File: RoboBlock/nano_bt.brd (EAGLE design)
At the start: 100 x 80 mm, 17 parts, among them IC1 L293D, M1 ARDUINO-NANO-3.0

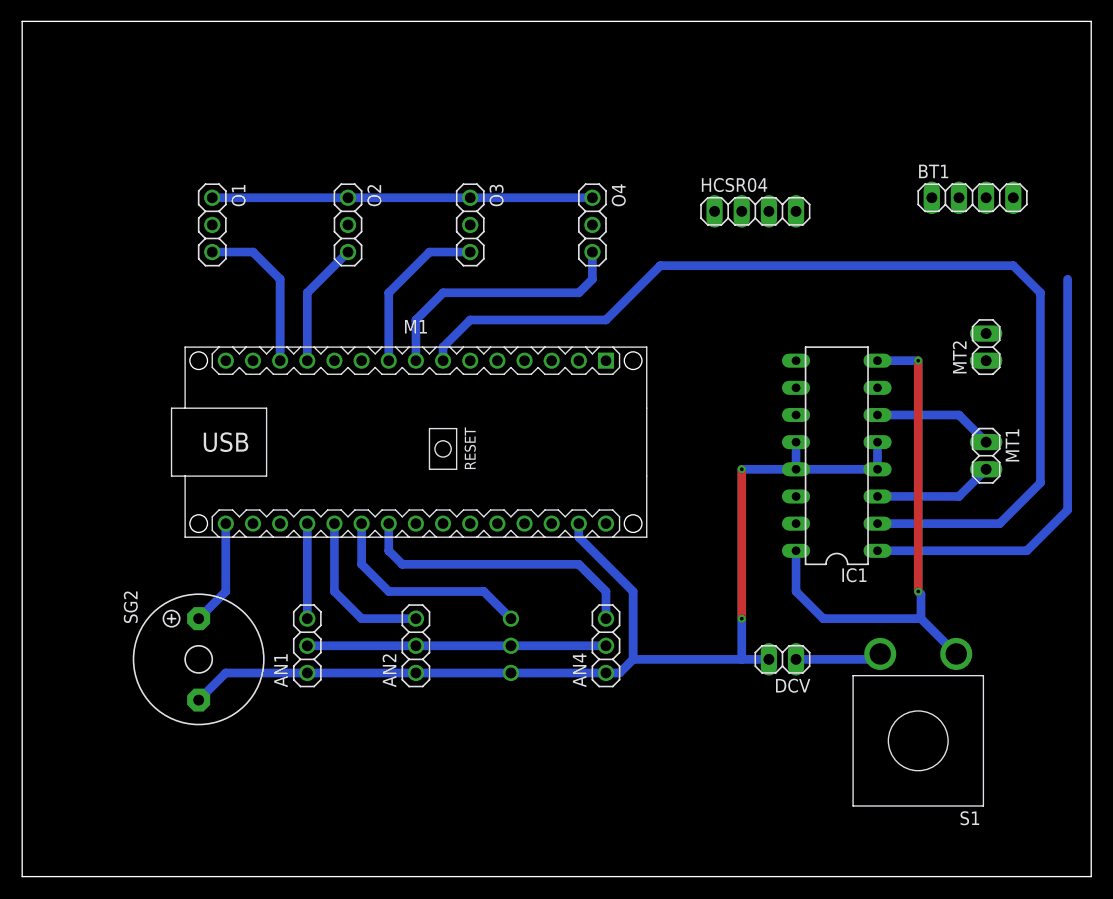
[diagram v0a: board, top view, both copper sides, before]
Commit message: printout pcb
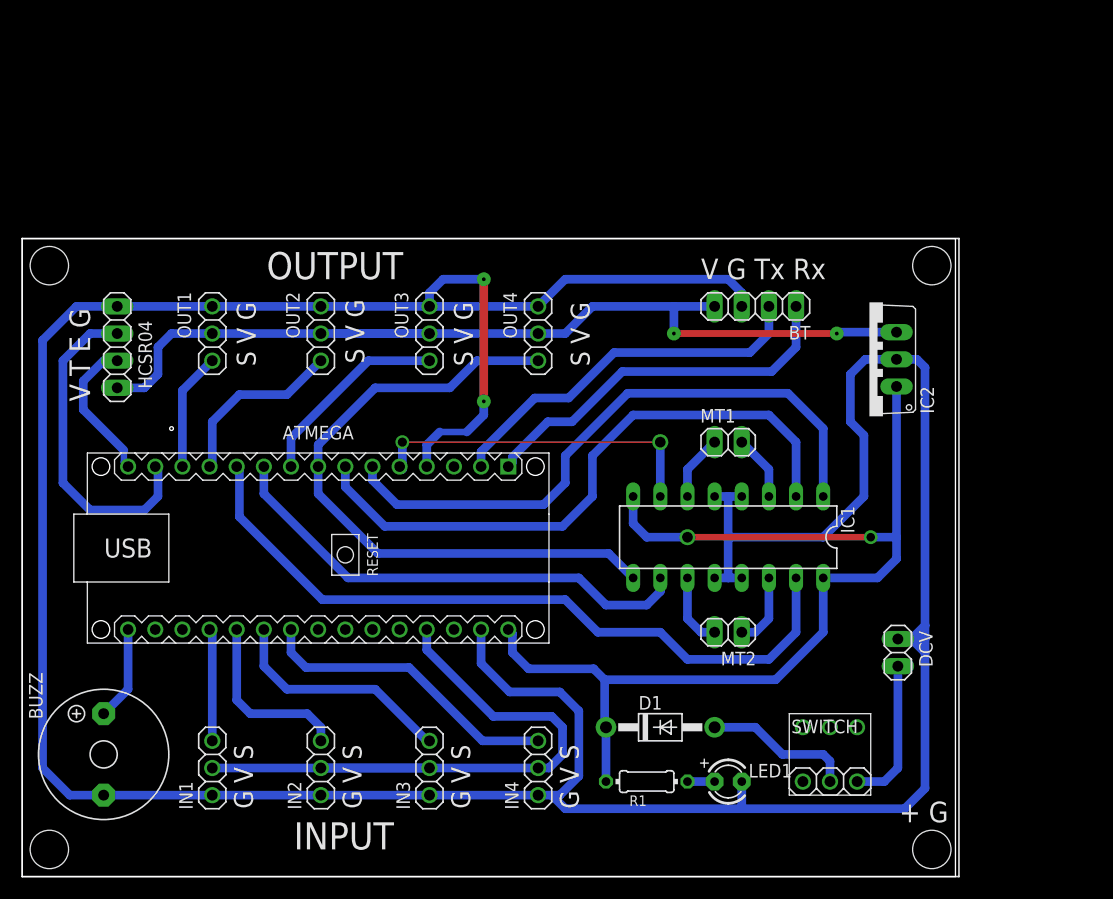
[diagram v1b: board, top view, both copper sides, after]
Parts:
- removed AN1, AN2, AN3, AN4, O1, O2, O3, O4: (no value), adafruit:1X03
- removed BT1: (no value), pinhead:1X04
- removed M1: ARDUINO-NANO-3.0, diy-modules:ARDUINO-NANO-3.0
- removed S1: SPST, adafruit_arduino:JUDCOSPST
- removed SG2: F/TMB, buzzer:F/TMB
- added ATMEGA: ARDUINO-NANO-3.0, diy-modules:ARDUINO-NANO-3.0
- added BT: (no value), pinhead:1X04
- added BUZZ: F/TMB, buzzer:F/TMB
- added D1: 1N4004, adafruit_arduino:DO41-10
- added IC2: 788TV, linear:TO220V
- added IN1, IN2, IN3, IN4, OUT1, OUT2, OUT3, OUT4: (no value), adafruit:1X03
- added LED1: (no value), adafruit_arduino:LED3MM
- added R1: 220, rcl:0204/7
- added SWITCH: (no value), adafruit_arduino:1X03
- moved HCSR04 61.0 mm to (8.89, 49.5), turned to 90 degrees
- moved MT2 36.0 mm to (66.0, 22.9), turned to 180 degrees
- moved MT1 24.2 mm to (66.0, 40.6), turned to 0 degrees
- moved IC1 12.7 mm to (66.0, 31.8), turned to 180 degrees
- moved DCV 10.8 mm to (81.9, 21.0), turned to 90 degrees
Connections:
- removed net 5V: M1.J2.4
- removed net VCC: AN1.2, AN2.2, AN3.2, AN4.2, BT1.4, HCSR04.1, O1.2, O2.2, O3.2, O4.2
- new net N$15: D1.A, SWITCH.2
- new net N$16: LED1.A, R1.1
- new net N$22: ATMEGA.J2.4, IN1.2, IN2.2, IN3.2, IN4.2
- new net VP: BT.4, HCSR04.1, IC2.3, OUT1.2, OUT2.2, OUT3.2, OUT4.2
- net 3V3: now also ATMEGA.J2.14; no longer M1.J2.14
- net A0: now also ATMEGA.J2.12, IN1.3; no longer AN1.3, M1.J2.12
- net A1: now also ATMEGA.J2.11, IN2.3; no longer AN2.3, M1.J2.11
- net A2: now also ATMEGA.J2.10, IN3.3; no longer AN3.3, M1.J2.10
- net A3: now also ATMEGA.J2.9, IN4.3; no longer AN4.3, M1.J2.9
- net EC: now also ATMEGA.J1.14; no longer M1.J1.14
- net GND: now also ATMEGA.J1.4, ATMEGA.J2.2, BT.3, BUZZ.-, IC2.2, IN1.1, IN2.1, IN3.1, IN4.1, LED1.K, OUT1.1, OUT2.1, OUT3.1, OUT4.1; no longer AN1.1, AN2.1, AN3.1, AN4.1, BT1.3, M1.J1.4, M1.J2.2, O1.1, O2.1, O3.1, O4.1, SG2.-
- net N$10: now also ATMEGA.J1.6; no longer M1.J1.6
- net N$11: now also ATMEGA.J1.7; no longer M1.J1.7
- net N$12: now also SWITCH.1; no longer S1.P
- net N$13: now also ATMEGA.J1.10; no longer M1.J1.10
- net N$14: now also ATMEGA.J1.11; no longer M1.J1.11
- net N$5: now also ATMEGA.J1.1, BT.1; no longer BT1.1, M1.J1.1
- net N$6: now also ATMEGA.J1.2, BT.2; no longer BT1.2, M1.J1.2
- net N$7: now also ATMEGA.J2.15, BUZZ.+; no longer M1.J2.15, SG2.+
- net N$8: now also ATMEGA.J2.1, D1.C, IC2.1, R1.2; no longer M1.J2.1, S1.T
- net N$9: now also ATMEGA.J1.5; no longer M1.J1.5
- net O1: now also ATMEGA.J1.13, OUT1.3; no longer M1.J1.13, O1.3
- net O2: now also ATMEGA.J1.12, OUT2.3; no longer M1.J1.12, O2.3
- net O3: now also ATMEGA.J1.9, OUT3.3; no longer M1.J1.9, O3.3
- net O4: now also ATMEGA.J1.8, OUT4.3; no longer M1.J1.8, O4.3
- net TR: now also ATMEGA.J1.15; no longer M1.J1.15
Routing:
- net GND: track 140.8 -> 340.8 mm
- net VP: track 0.00 -> 93.2 mm, vias 0 -> 2
- net N$14: track 0.00 -> 68.5 mm
- net N$22: track 0.00 -> 63.6 mm
- net N$8: track 49.3 -> 100.4 mm
- net N$13: track 0.00 -> 45.7 mm
- net N$11: track 96.0 -> 58.3 mm
- net O4: track 24.4 -> 61.1 mm
- net N$5: track 0.00 -> 35.7 mm
- net N$6: track 0.00 -> 35.4 mm
- net N$9: track 0.00 -> 32.1 mm, vias 0 -> 2
- net EC: track 0.00 -> 30.9 mm
- net VCC: track 27.9 -> 0.00 mm
- net N$10: track 40.9 -> 57.9 mm
- net N$15: track 0.00 -> 14.0 mm
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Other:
- board size 100 x 80 mm -> 87.3 x 59.7 mm
- board text added: "+ G"
- board text added: "G V S"
- board text added: "INPUT"
- board text added: "OUTPUT"
- board text added: "S V G"
- board text added: "V G Tx Rx"
- board text added: "V T E G"
